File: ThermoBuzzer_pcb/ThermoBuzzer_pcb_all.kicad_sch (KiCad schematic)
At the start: 21 parts, among them SW1 SW_Push, SW2 SW_Push

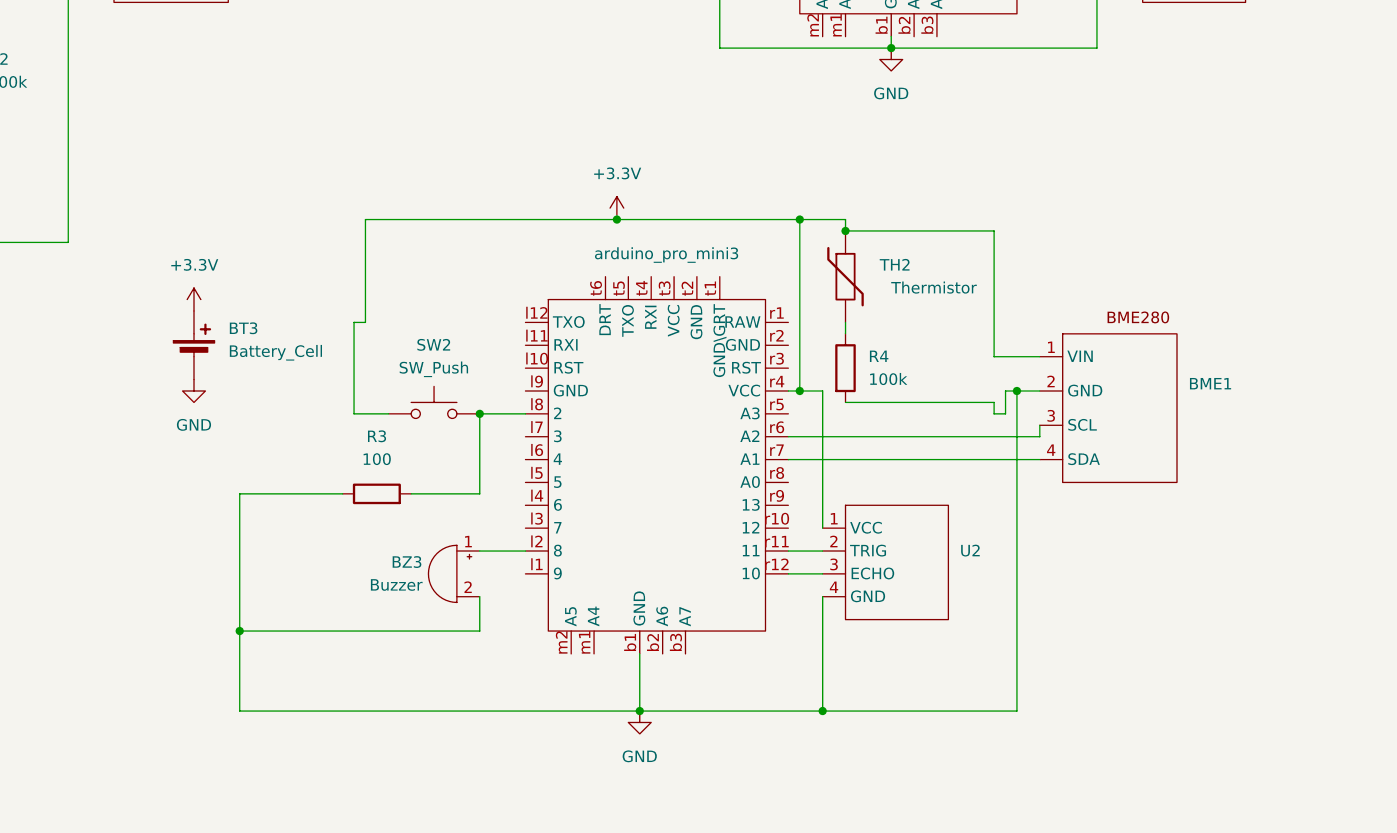
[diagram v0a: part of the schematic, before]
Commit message: 4.21
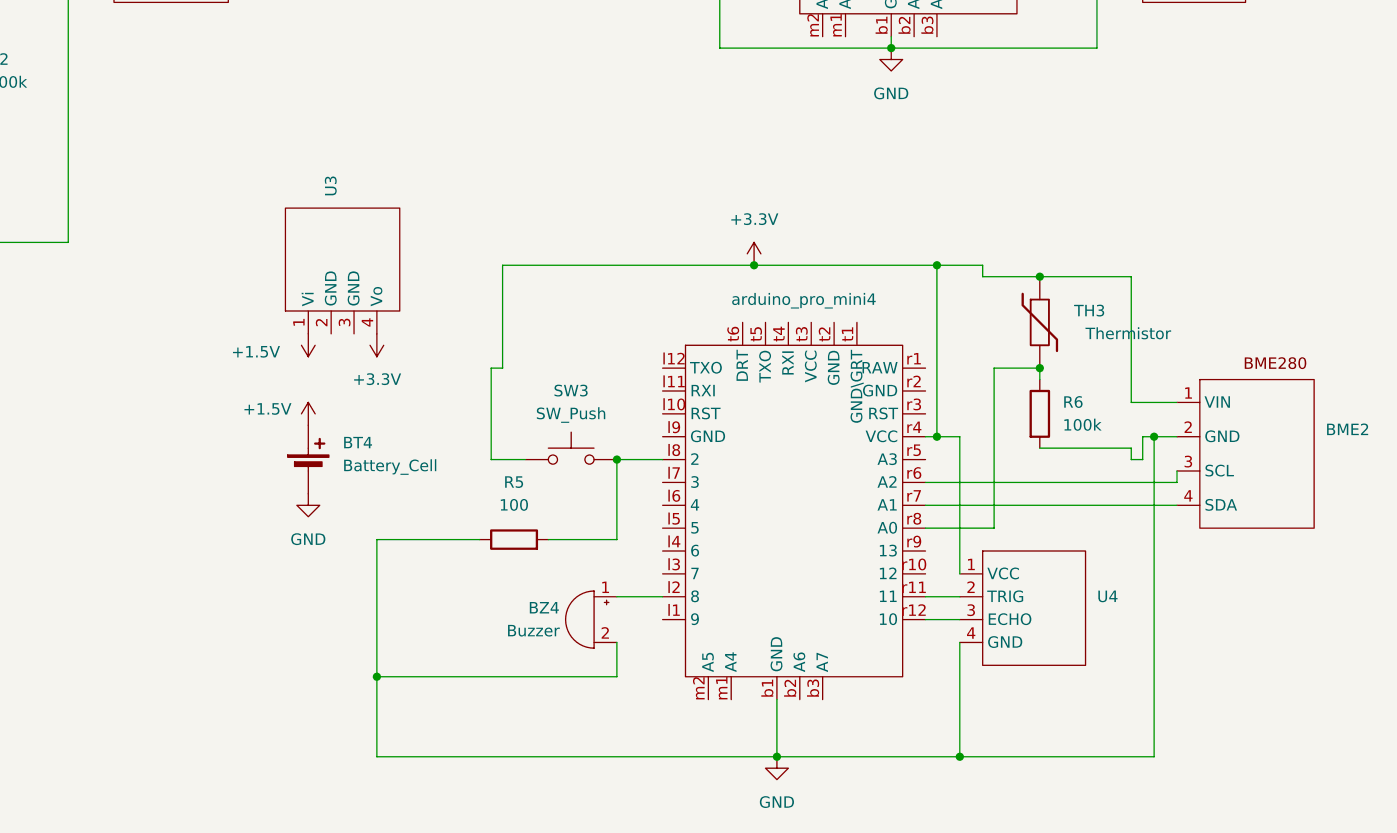
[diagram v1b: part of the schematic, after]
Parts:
- removed BME1: ~, custom_footprints:AHT20+BMP280, symbol thermosensor:BME280_new
- removed BT3: Battery_Cell, Resistor_THT:R_Axial_DIN0204_L3.6mm_D1.6mm_P1.90mm_Vertical, symbol Device:Battery_Cell
- removed BZ3: Buzzer, Buzzer_Beeper:Buzzer_12x9.5RM7.6, symbol Device:Buzzer
- removed R3: 100, Resistor_THT:R_Axial_DIN0207_L6.3mm_D2.5mm_P7.62mm_Horizontal, symbol Device:R
- removed R4: 100k, Resistor_THT:R_Axial_DIN0207_L6.3mm_D2.5mm_P7.62mm_Horizontal, symbol Device:R
- removed SW2: SW_Push, Button_Switch_THT:SW_PUSH_6mm, symbol Switch:SW_Push
- removed TH2: Thermistor, Resistor_THT:R_Axial_DIN0207_L6.3mm_D2.5mm_P7.62mm_Horizontal, symbol Device:Thermistor
- removed U2: ~, symbol thermosensor:HC-SR04
- removed arduino_pro_mini3: ~, custom_footprints:arduino_pro_mini_new, symbol thermosensor:Arduino_pro_mini
- added BME2: ~, custom_footprints:AHT20+BMP280, symbol thermosensor:BME280_new
- added BT4: Battery_Cell, Battery:BatteryHolder_Keystone_2460_1xAA, symbol Device:Battery_Cell
- added BZ4: Buzzer, Buzzer_Beeper:Buzzer_12x9.5RM7.6, symbol Device:Buzzer
- added R5: 100, Resistor_THT:R_Axial_DIN0207_L6.3mm_D2.5mm_P7.62mm_Horizontal, symbol Device:R
- added R6: 100k, Resistor_THT:R_Axial_DIN0207_L6.3mm_D2.5mm_P7.62mm_Horizontal, symbol Device:R
- added SW3: SW_Push, Button_Switch_THT:SW_PUSH_6mm, symbol Switch:SW_Push
- added TH3: Thermistor, Resistor_THT:R_Axial_DIN0207_L6.3mm_D2.5mm_P7.62mm_Horizontal, symbol Device:Thermistor
- added U3: ~, custom_footprints:ND0205MA Voltage Regulator, symbol thermosensor:ND0205MA_Voltage_Regulator
- added U4: ~, custom_footprints:Ultrasonic Sensor HC-SR04, symbol thermosensor:HC-SR04
- added arduino_pro_mini4: ~, custom_footprints:arduino_pro_mini_new, symbol thermosensor:Arduino_pro_mini
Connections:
- net +3.3V: now also BME2.1 (VIN), SW3.1, TH3.1, U3.4 (Vo), U4.1 (VCC), arduino_pro_mini4.r4 (VCC)
- net GND: now also BME2.2 (GND), BT4.2 (-), BZ4.2 (-), R5.1, R6.2, U4.4 (GND), arduino_pro_mini4.b1 (GND)
- new net: BME2.3 (SCL), arduino_pro_mini4.r6 (A2)
- new net: BME2.4 (SDA), arduino_pro_mini4.r7 (A1)
- new net: R6.1, TH3.2, arduino_pro_mini4.r8 (A0)
- new net: BZ4.1 (+), arduino_pro_mini4.l2 (8)
- new net: R5.2, SW3.2, arduino_pro_mini4.l8 (2)
- new net: U4.2 (TRIG), arduino_pro_mini4.r11 (11)
- new net: U4.3 (ECHO), arduino_pro_mini4.r12 (10)
- new net +1.5V: BT4.1 (+), U3.1 (Vi)
